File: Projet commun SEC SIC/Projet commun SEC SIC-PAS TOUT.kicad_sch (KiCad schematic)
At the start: 10 parts, among them J1 Conn_01x08_Female, J2 Conn_01x06_Female, J3 Conn_01x09_Female, U1 ATmega328-P, U2 LM1117-5.0, Y1 Crystal

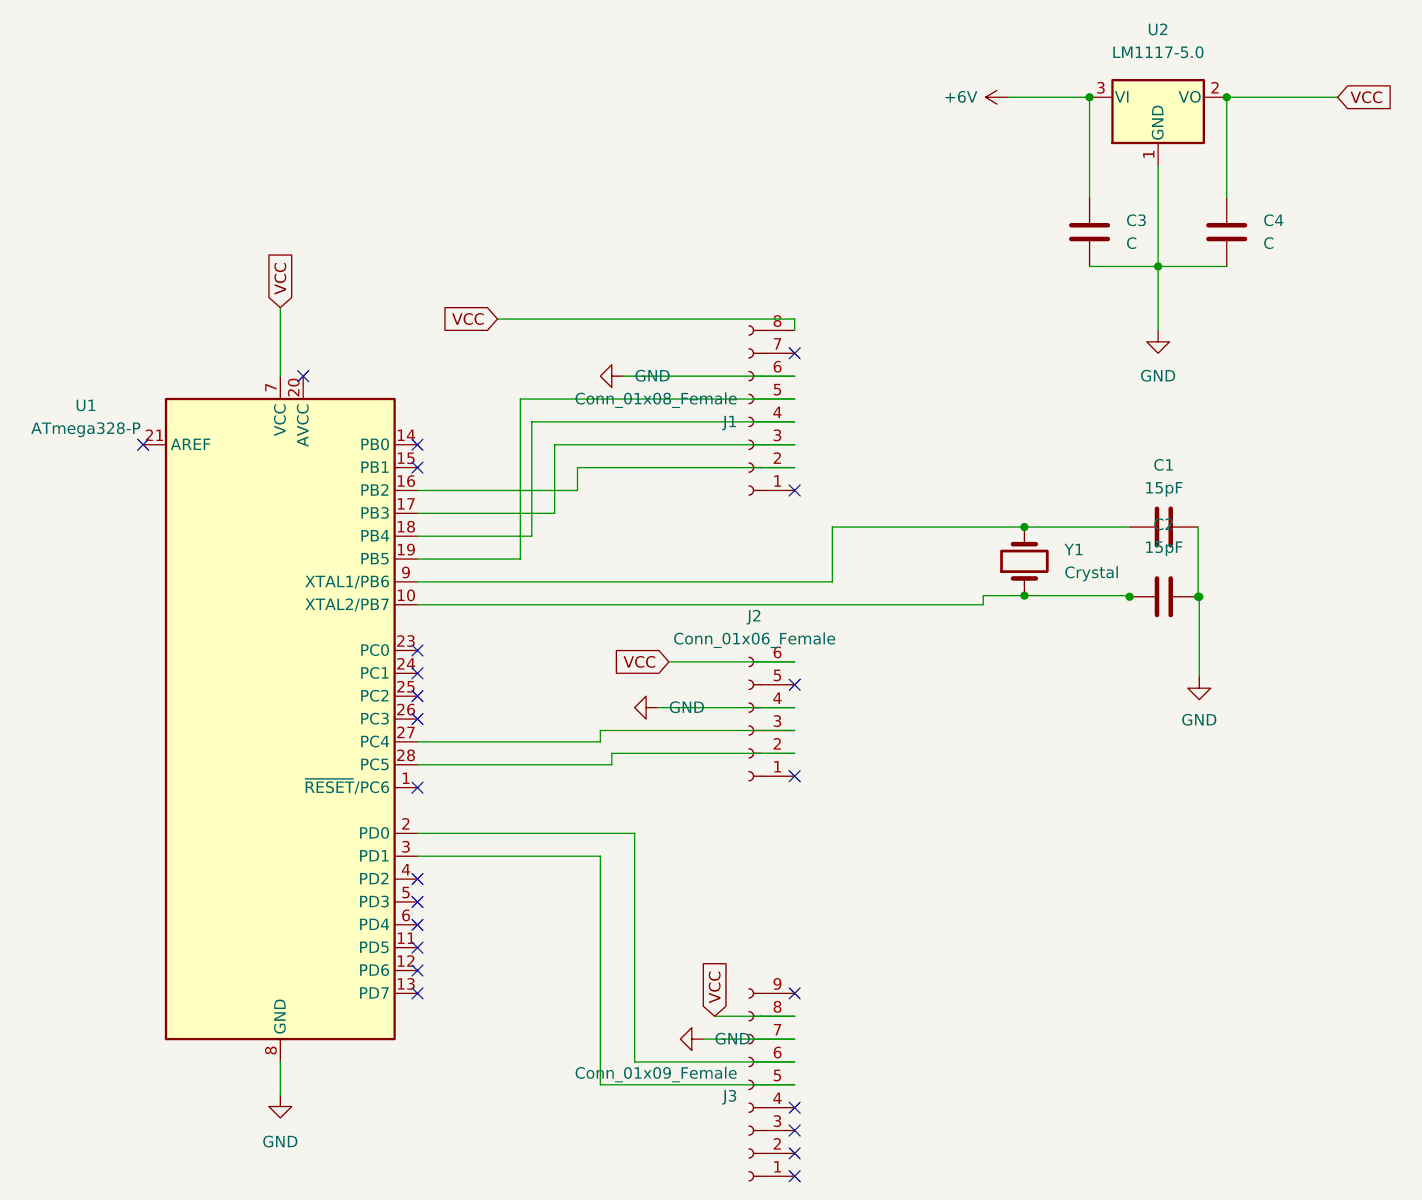
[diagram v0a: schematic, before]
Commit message: PCB fini
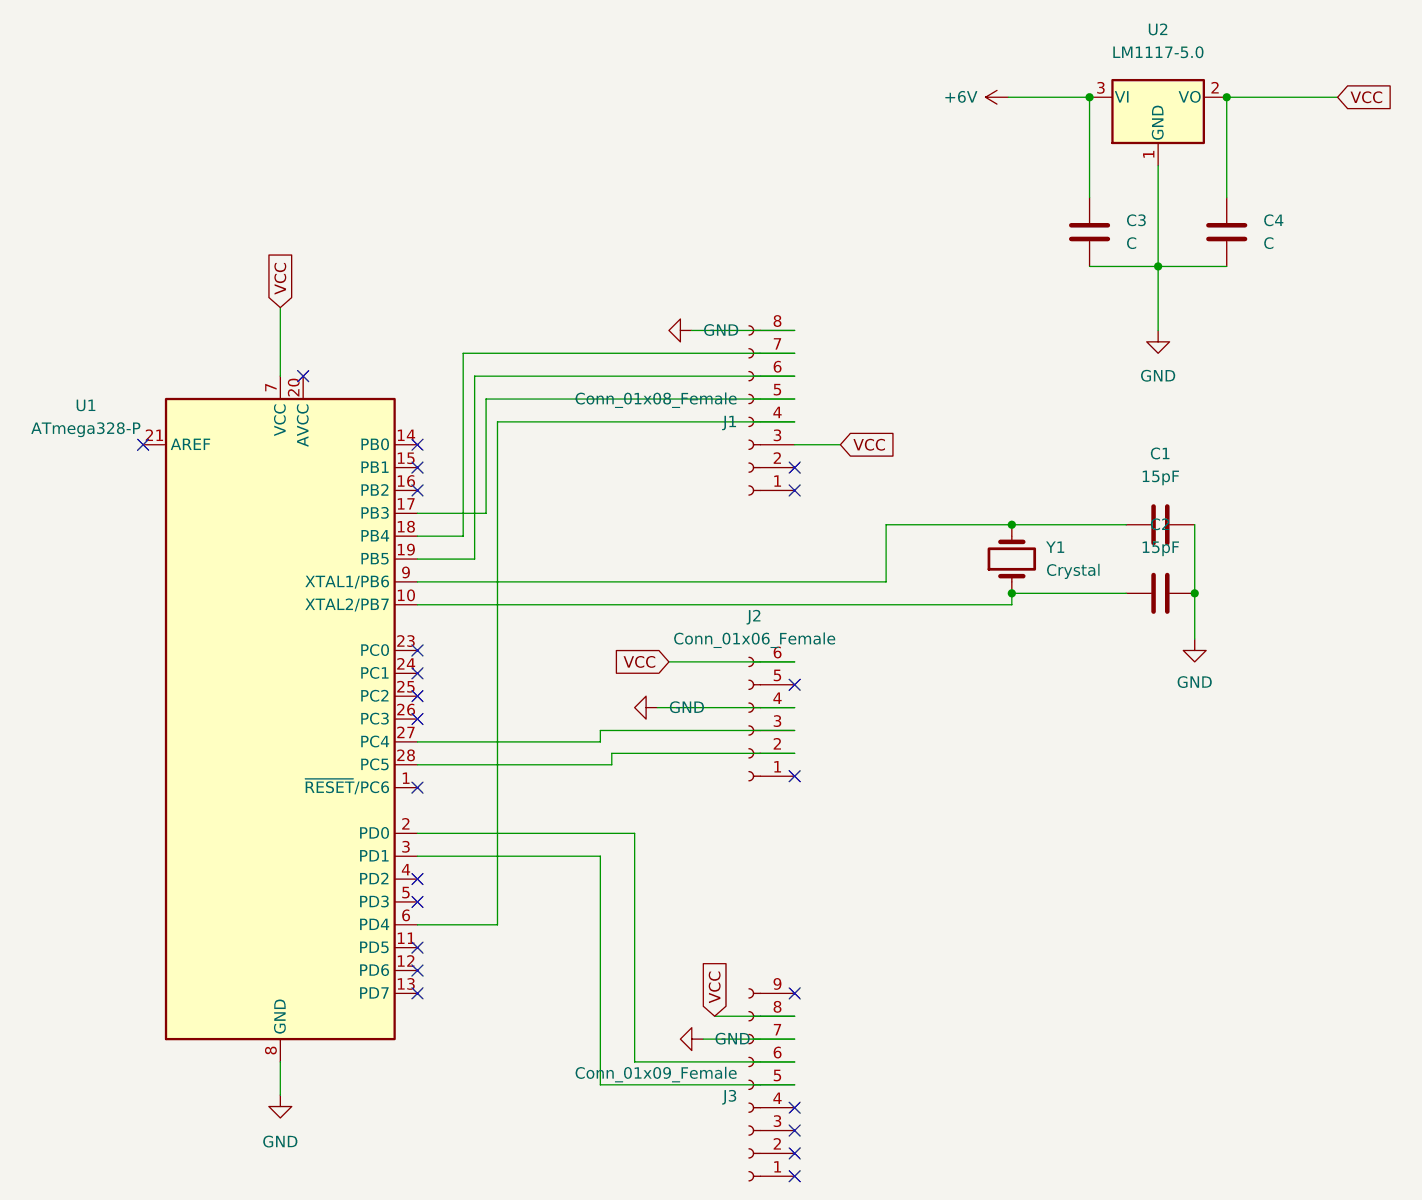
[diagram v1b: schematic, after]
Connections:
- net GND: now also C1.1, C2.1, J1.8 (Pin_8); no longer C1.2, C2.2, J1.6 (Pin_6)
- net VCC: now also J1.3 (Pin_3); no longer J1.8 (Pin_8)
- net at U1.10 (XTAL2/PB7), Y1.1: now also C2.2; no longer C2.1
- net at U1.16 (PB2): no longer J1.2 (Pin_2)
- net at U1.17 (PB3): now also J1.5 (Pin_5); no longer J1.3 (Pin_3)
- net at U1.18 (PB4): now also J1.7 (Pin_7); no longer J1.4 (Pin_4)
- net at U1.19 (PB5): now also J1.6 (Pin_6); no longer J1.5 (Pin_5)
- net at U1.6 (PD4): now also J1.4 (Pin_4)
- net at U1.9 (XTAL1/PB6), Y1.2: now also C1.2; no longer C1.1
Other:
- moved on the sheet: C1, C2
